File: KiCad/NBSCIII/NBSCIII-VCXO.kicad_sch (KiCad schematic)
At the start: 20 parts, among them Q1000 BC337-25, Q1001 2SC1906, X1000 6.000Mhz HC49/U

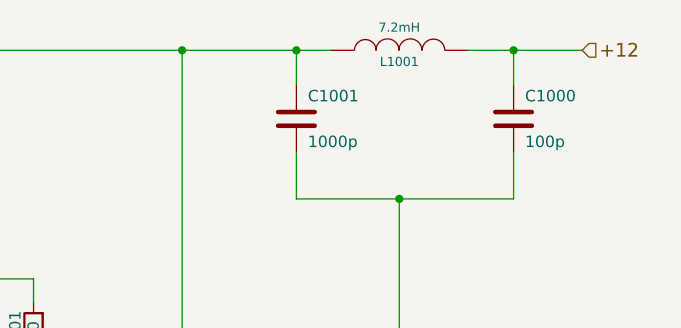
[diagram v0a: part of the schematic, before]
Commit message: unrescue Device:L_small
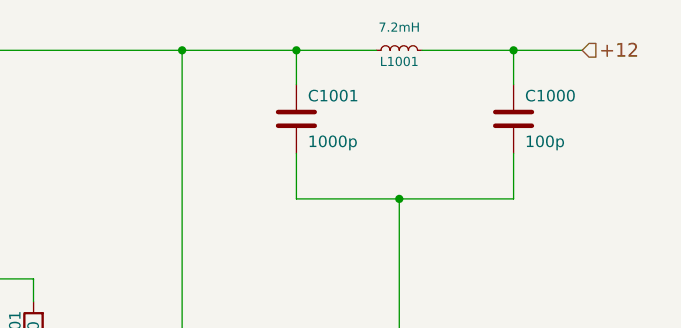
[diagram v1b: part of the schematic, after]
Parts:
- L1001: symbol NBSCIII-rescue:INDUCTOR -> Device:L_Small
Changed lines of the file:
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@@
     (stroke (width 0) (type default) (color 0 0 0 0))
   )
-  (wire (pts (xy 199.39 54.61) (xy 195.58 54.61))
+  (wire (pts (xy 195.58 54.61) (xy 204.47 54.61))
     (stroke (width 0) (type default) (color 0 0 0 0))
   )
-  (wire (pts (xy 214.63 54.61) (xy 219.71 54.61))
+  (wire (pts (xy 209.55 54.61) (xy 219.71 54.61))
     (stroke (width 0) (type default) (color 0 0 0 0))
   )
@@
     (effects (font (size 1.524 1.524)) (justify left))
   )
-  (symbol (lib_id "NBSCIII-rescue:INDUCTOR") (at 207.01 54.61 90) (unit 1)
+  (symbol (lib_id "Device:L_Small") (at 207.01 54.61 90) (unit 1)
     (in_bom yes) (on_board yes)
     (property "Reference" "L1001" (id 0) (at 207.01 55.88 90)
